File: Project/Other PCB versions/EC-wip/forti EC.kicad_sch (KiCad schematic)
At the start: 27 parts, among them J1 USB_C_Receptacle_USB2.0, SW38 BOOT0, U1 STM32F401CBUx, U2 USBLC6-2SC6, U4 XC6206PxxxMR-Regulator_Linear, Y1 8 MHz

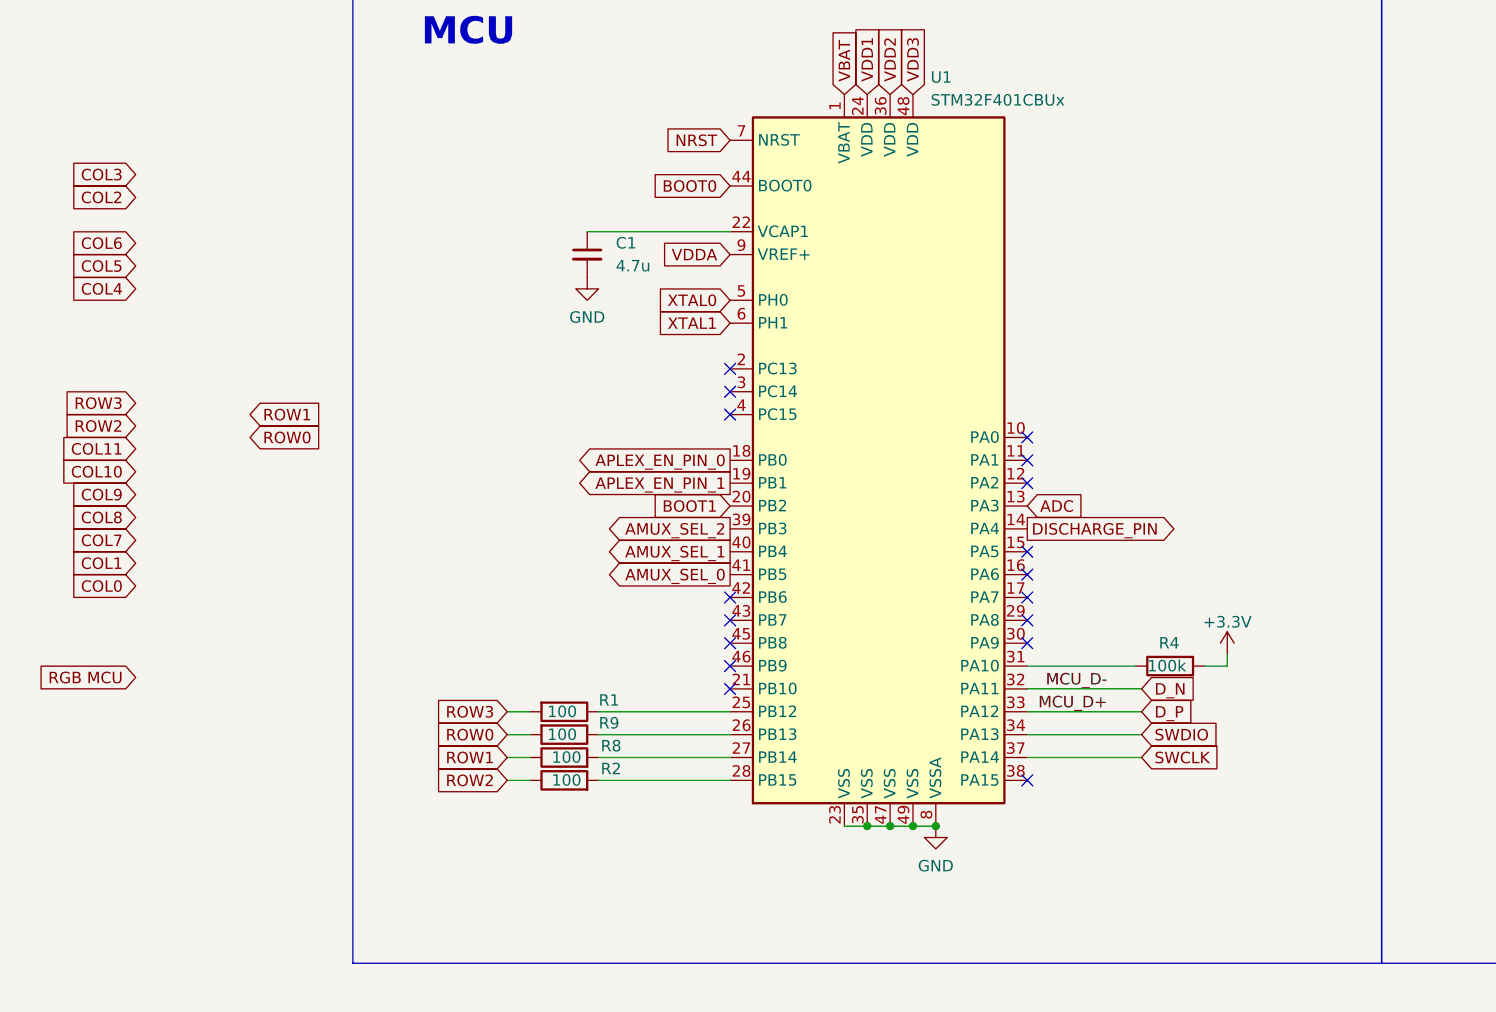
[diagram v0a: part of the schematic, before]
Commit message: EC progress
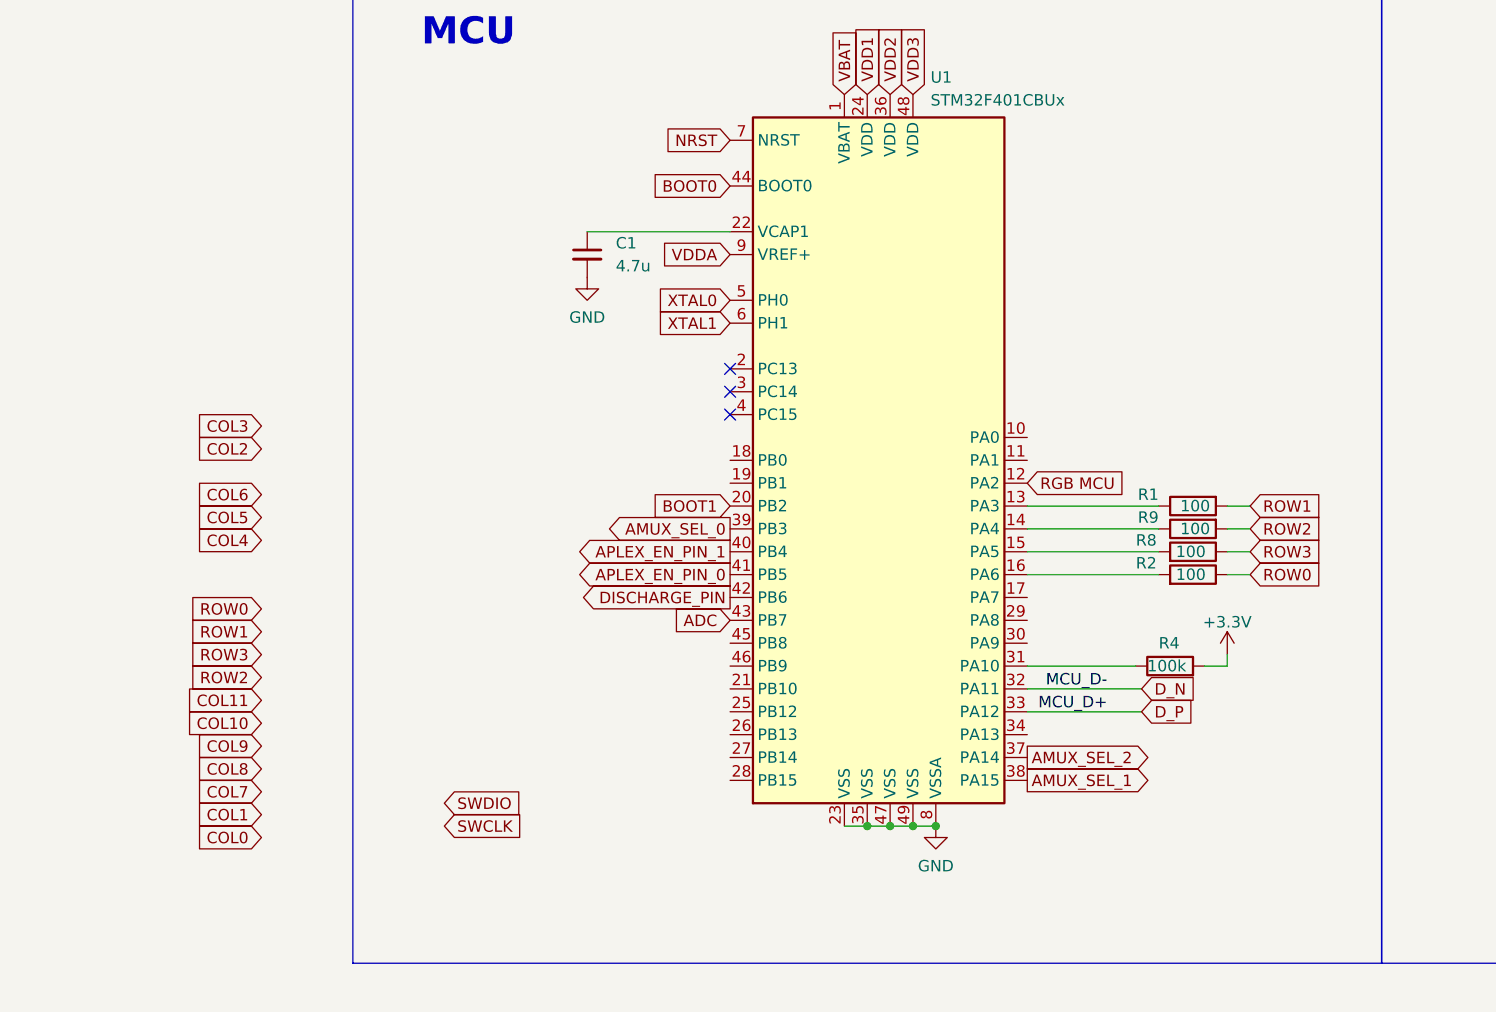
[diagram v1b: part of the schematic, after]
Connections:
- net ADC: now also U1.43 (PB7); no longer U1.13 (PA3)
- net AMUX_SEL_0: now also U1.39 (PB3); no longer U1.41 (PB5)
- net AMUX_SEL_1: now also U1.38 (PA15); no longer U1.40 (PB4)
- net AMUX_SEL_2: now also U1.37 (PA14); no longer U1.39 (PB3)
- net APLEX_EN_PIN_0: now also U1.41 (PB5); no longer U1.18 (PB0)
- net APLEX_EN_PIN_1: now also U1.40 (PB4); no longer U1.19 (PB1)
- net DISCHARGE_PIN: now also U1.42 (PB6); no longer U1.14 (PA4)
- net RGB MCU: now also U1.12 (PA2)
- net ROW0: now also R2.1; no longer R9.2
- net ROW1: now also R1.2; no longer R8.1
- net ROW2: now also R9.2; no longer R2.1
- net ROW3: now also R8.1; no longer R1.2
- net SWCLK: no longer U1.37 (PA14)
- net SWDIO: no longer U1.34 (PA13)
- net at U1.15 (PA5): now also R8.2
- net at U1.16 (PA6): now also R2.2
- net at R1.1: now also U1.13 (PA3); no longer U1.25 (PB12)
- net at R9.1: now also U1.14 (PA4); no longer U1.26 (PB13)
- net at U1.27 (PB14): no longer R8.2
- net at U1.28 (PB15): no longer R2.2
- no-connect marks 19 -> 5
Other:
- moved on the sheet: R1, R2, R8, R9
